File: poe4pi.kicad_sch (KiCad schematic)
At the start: 24 parts, among them J1 Conn_02x02_Odd_Even, J2 Conn_02x02_Odd_Even, J3 Conn_02x20_Odd_Even, U1 LTC4413EDD-2-PBF, U3 TPS2375-1

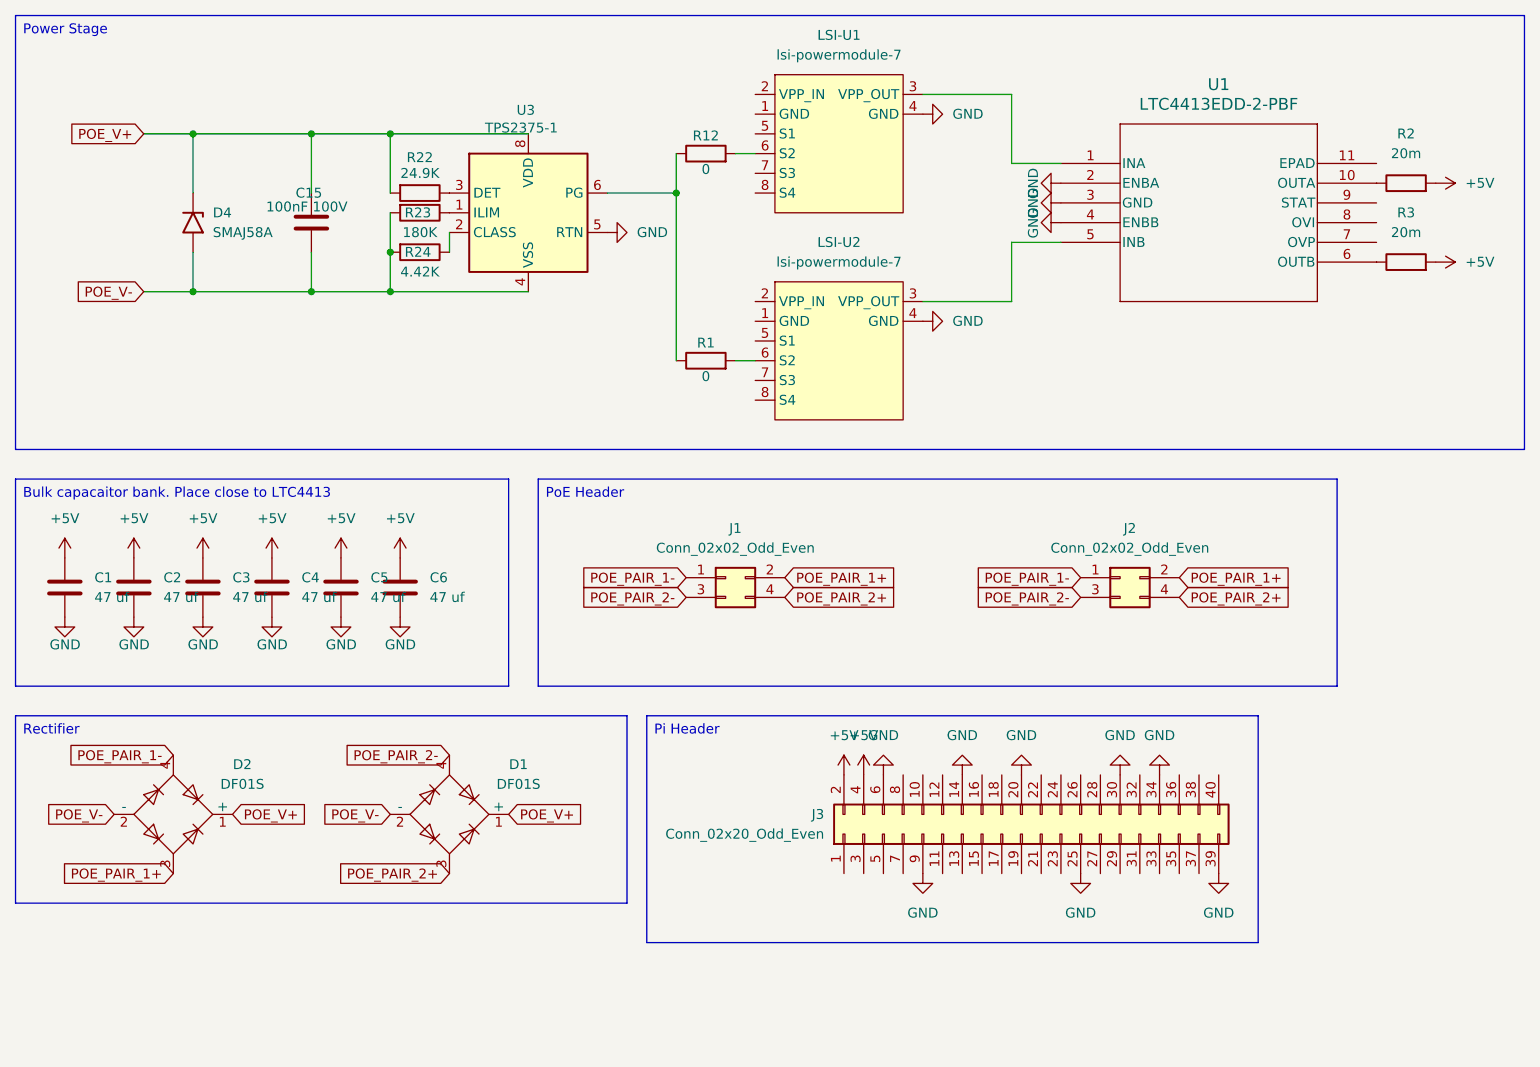
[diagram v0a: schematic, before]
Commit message: feat: header placement
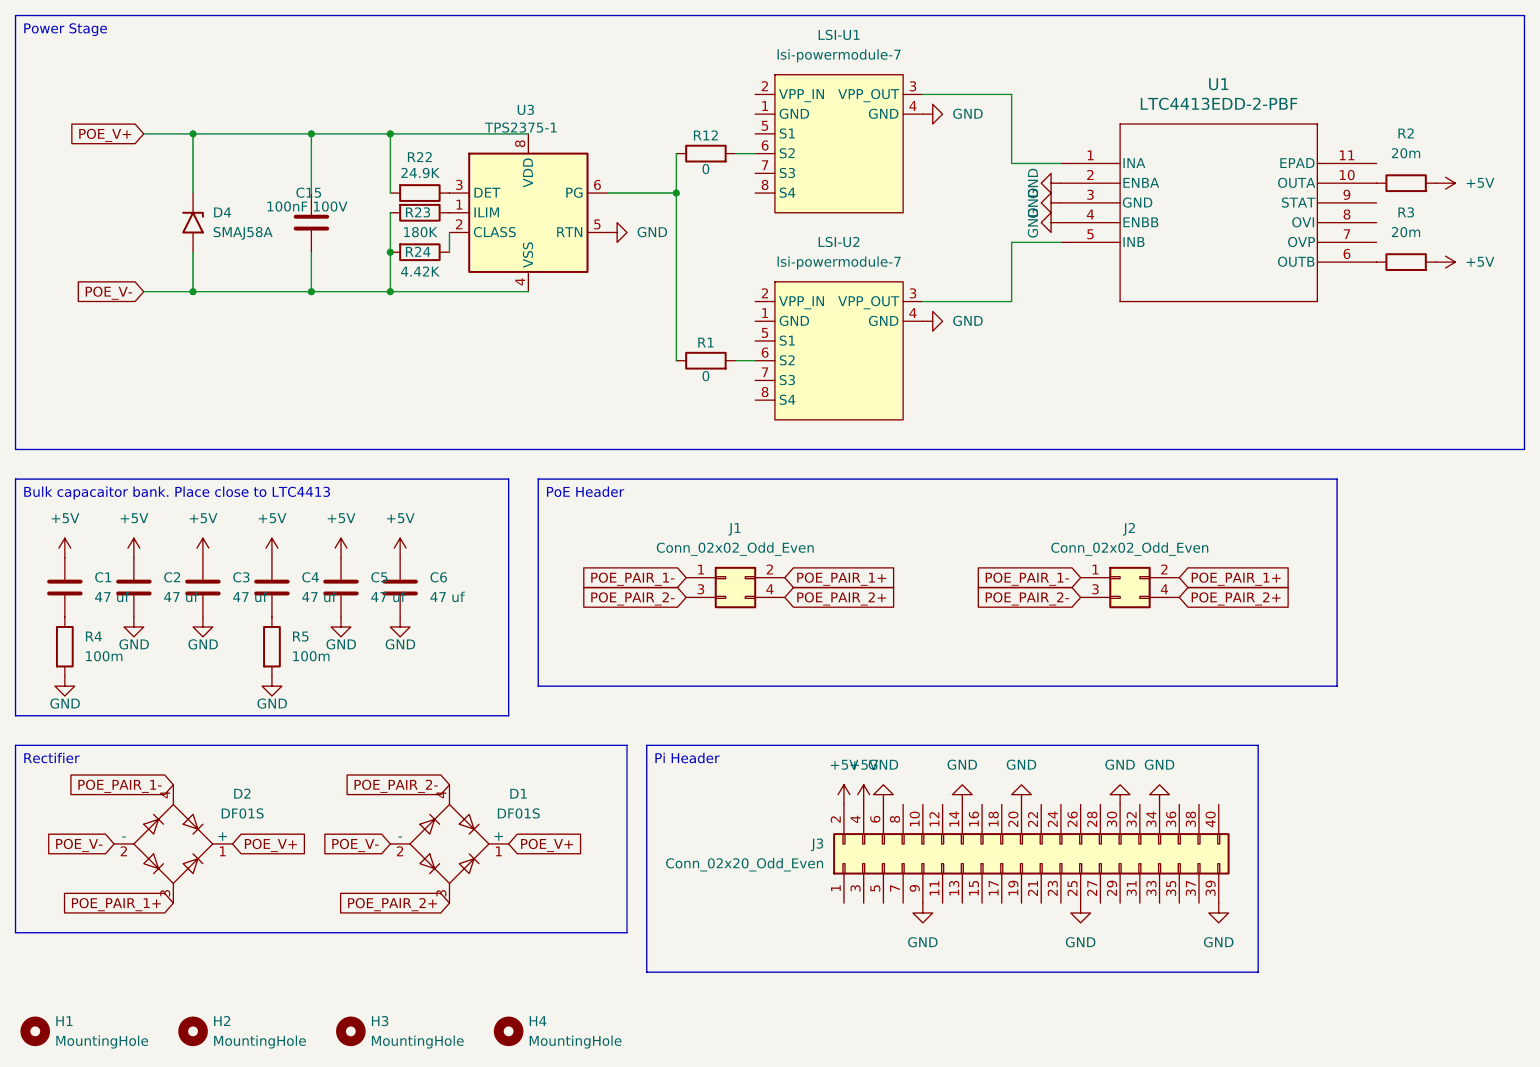
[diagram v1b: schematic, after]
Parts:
- added H1, H2, H3, H4: MountingHole, MountingHole:MountingHole_2.5mm, symbol Mechanical:MountingHole
- added R4, R5: 100m, Resistor_SMD:R_1210_3225Metric, symbol Device:R
- D1, D2: footprint Diode_THT:Diode_Bridge_Round_D9.8mm -> Diode_SMD:Diode_Bridge_OnSemi_SDIP-4L
- J1, J2: footprint Connector_PinSocket_1.27mm:PinSocket_2x02_P1.27mm_Vertical -> Connector_PinSocket_2.54mm:PinSocket_2x02_P2.54mm_Vertical
- J3: footprint (none) -> Connector_PinHeader_2.54mm:PinHeader_2x20_P2.54mm_Vertical
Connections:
- net GND: now also R4.2, R5.2; no longer C1.2, C4.2
- new net: C4.2, R5.1
- new net: C1.2, R4.1
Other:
- moved on the sheet: D1, D2
